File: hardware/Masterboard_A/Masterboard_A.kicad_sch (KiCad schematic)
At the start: 29 parts, among them J1 Conn_01x09_Socket, J102 Conn_01x09_Socket, J102 Conn_02x05_Odd_Even, J2 Conn_02x05_Odd_Even, J3 Conn_01x04_Pin, SW1 SW_Push, U2 MCU-MSM0G3507SPM

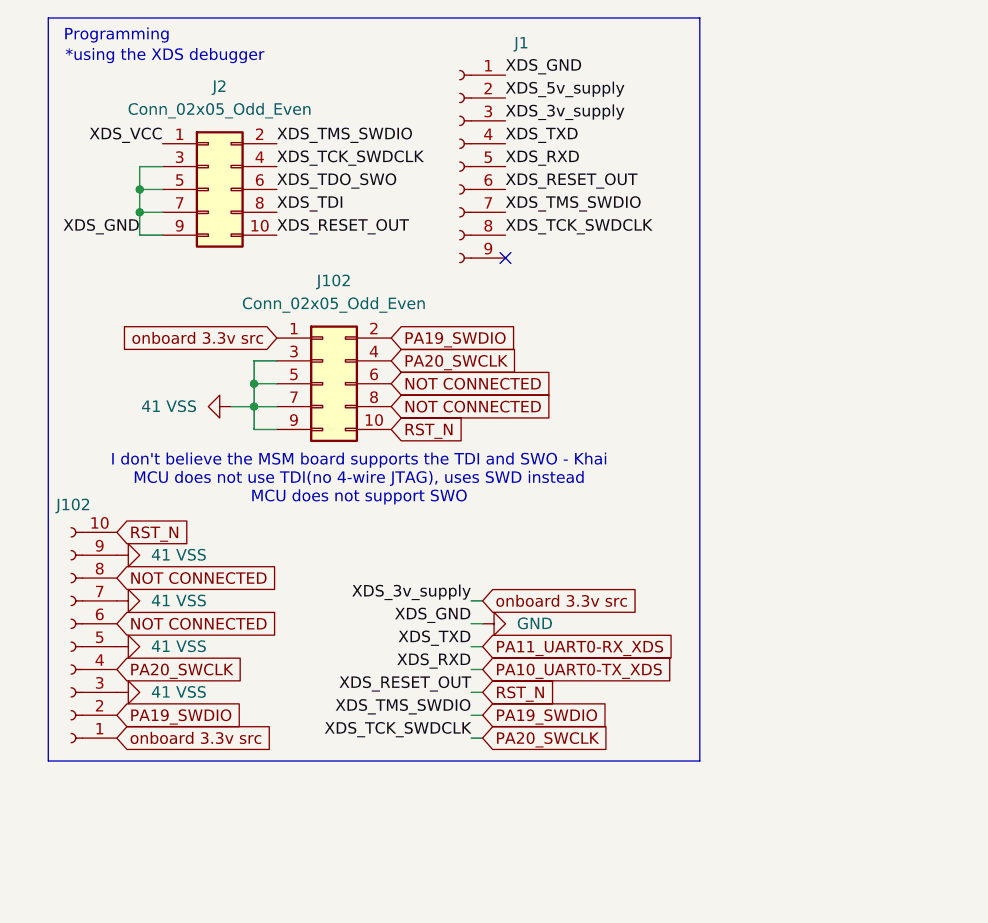
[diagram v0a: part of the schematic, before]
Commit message: changed
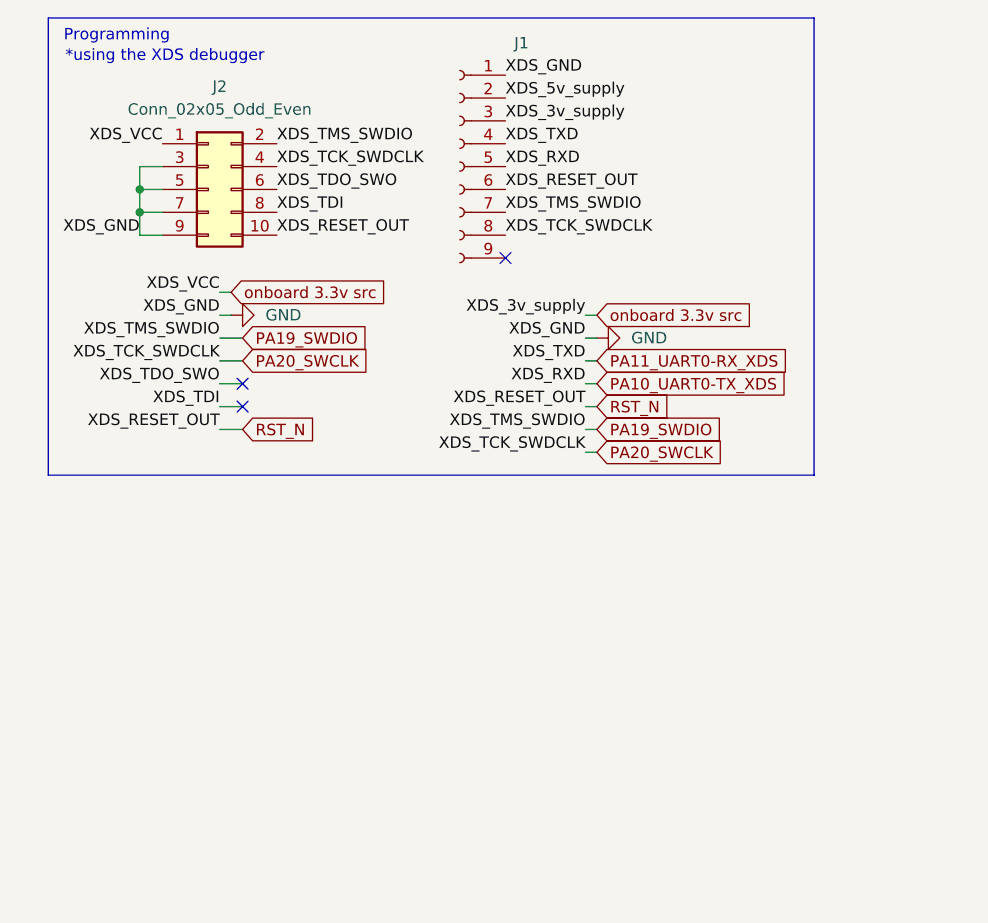
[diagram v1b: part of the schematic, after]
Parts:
- removed J102: Conn_01x09_Socket, Connector_PinHeader_2.54mm:PinHeader_1x09_P2.54mm_Vertical, symbol Connector:Conn_01x09_Socket
- removed J102: Conn_02x05_Odd_Even, Connector_PinHeader_1.27mm:PinHeader_2x05_P1.27mm_Vertical_SMD, symbol Connector_Generic:Conn_02x05_Odd_Even
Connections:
- net XDS_VCC is gone; now on net onboard 3.3v src: J2.1 (Pin_1)
- no-connect marks 45 -> 47
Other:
- note removed: "I don't believe the MSM board supports the TDI and SWO - Khai MCU does not use TDI(no 4-wire JTAG), uses SWD instead MCU does not support SWO"
